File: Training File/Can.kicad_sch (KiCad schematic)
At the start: 7 parts, among them U2 OKI

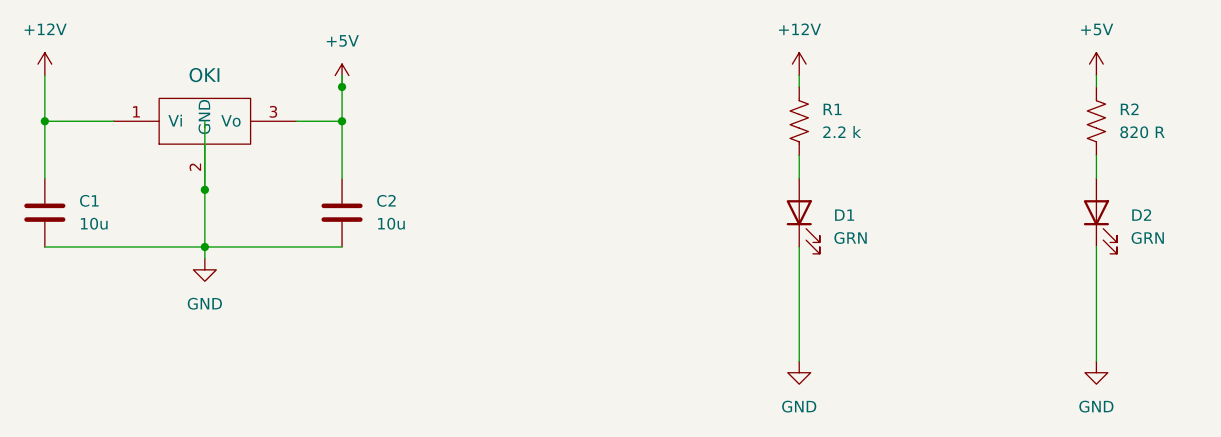
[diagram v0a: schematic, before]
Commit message: CAN reciever
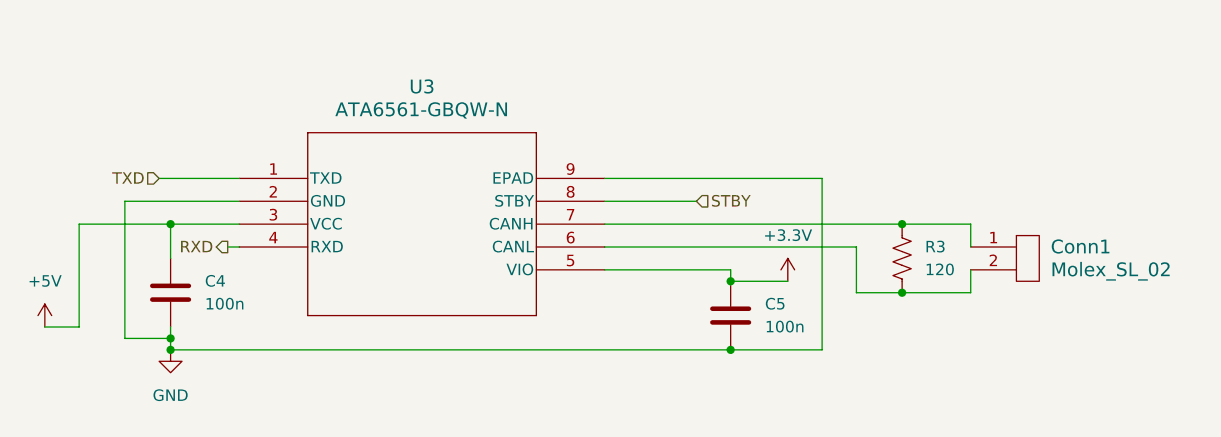
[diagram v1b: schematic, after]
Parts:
- removed C1, C2: 10u, symbol Device:C
- removed D1, D2: GRN, symbol Device:LED
- removed R1: 2.2 k, symbol Device:R_US
- removed R2: 820 R, symbol Device:R_US
- removed U2: OKI, symbol MRDT_Devices:OKI
- added C4, C5: 100n, symbol Device:C
- added Conn1: Molex_SL_02, symbol MRDT_Connectors:Molex_SL_02
- added R3: 120, symbol Device:R_US
- added U3: ATA6561-GBQW-N, VDFN8_3X3_MCH, symbol 2026_training_lib:ATA6561-GBQW-N
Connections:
- net +5V: now also C4.1, U3.3 (VCC)
- net GND: now also C4.2, C5.2, U3.2 (GND), U3.9 (EPAD)
- new net: Conn1.1, R3.1, U3.7 (CANH)
- new net: Conn1.2, R3.2, U3.6 (CANL)
- new net +3.3V: C5.1, U3.5 (VIO)
- new net RXD: U3.4 (RXD)
- new net STBY: U3.8 (STBY)
- new net TXD: U3.1 (TXD)
